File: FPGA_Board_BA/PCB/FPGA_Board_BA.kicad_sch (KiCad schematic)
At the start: 0 parts

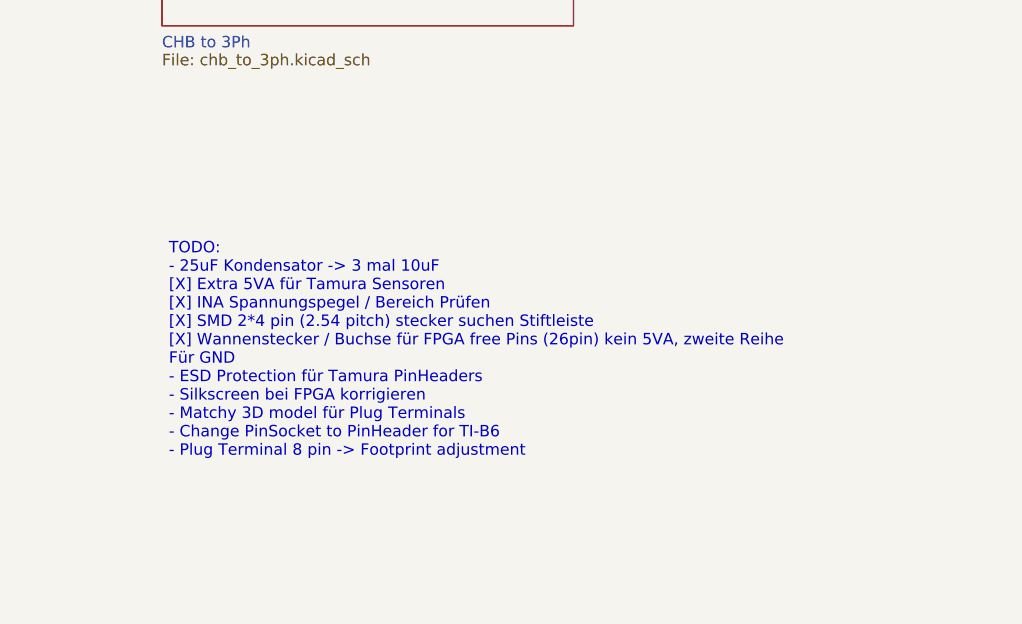
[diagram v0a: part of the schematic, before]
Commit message: Component placement ready. Waiting to meet with Leo
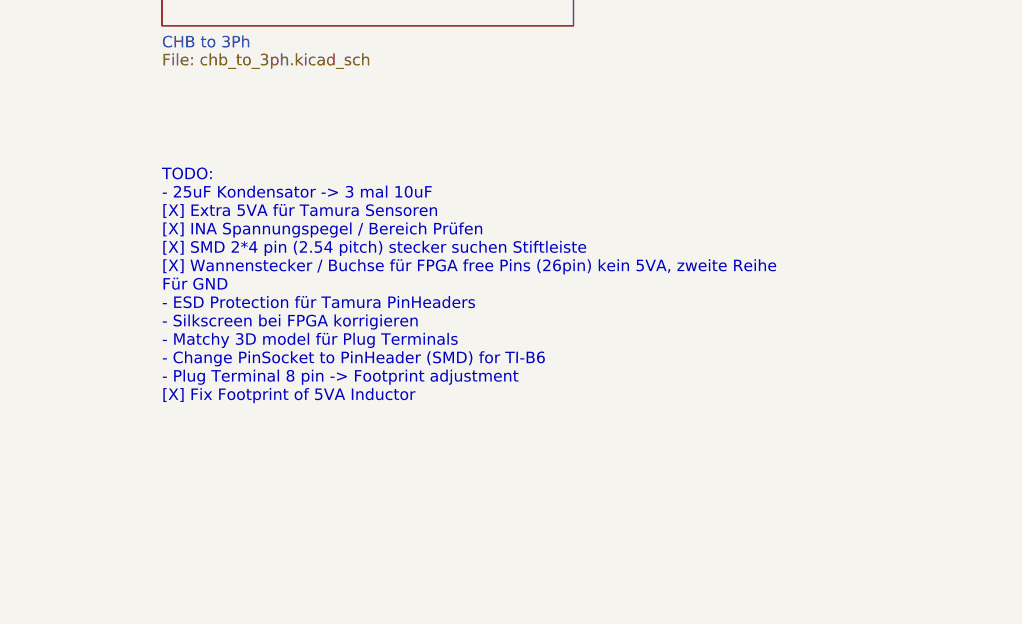
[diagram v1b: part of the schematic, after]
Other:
- note added: "TODO: - 25uF Kondensator -> 3 mal 10uF [X] Extra 5VA für Tamura Sensoren [X] INA Spannungspegel / Bereich Prüfen [X] SMD 2*4 pin (2.54 pitch) stecker suchen Stiftleiste [X] Wannenstecker / Buchse für FPGA free Pins (26pin) kein 5VA, zweite Reihe Für GND - ESD Protection für Tamura PinHeaders - Silkscreen bei FPGA korrigieren - Matchy 3D model für Plug Terminals - Change PinSocket to PinHeader (SM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"
- note removed: "TODO: - 25uF Kondensator -> 3 mal 10uF [X] Extra 5VA für Tamura Sensoren [X] INA Spannungspegel / Bereich Prüfen [X] SMD 2*4 pin (2.54 pitch) stecker suchen Stiftleiste [X] Wannenstecker / Buchse für FPGA free Pins (26pin) kein 5VA, zweite Reihe Für GND - ESD Protection für Tamura PinHeaders - Silkscreen bei FPGA korrigieren - Matchy 3D model für Plug Terminals - Change PinSocket to PinHeader for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"
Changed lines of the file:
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@@
 	(generator_version "9.0")
 	(paper "A3")
-	(text "TODO:\n- 25uF Kondensator -> 3 mal 10uF \n[X] Extra 5VA für Tamura Sensoren\n[X] INA Spannungspegel / Bereich Prüfen\n[X] SMD 2*4 pin (2.54 pitch) stecker suchen Stiftleiste\n[X] Wannenstecker / Buchse für FPGA free Pins (26pin) kein 5VA, zweite Reihe\nFür GND\n- ESD Protection für Tamura PinHeaders\n- Silkscreen bei FPGA korrigieren\n- Matchy 3D model für Plug Terminals\n- Change PinSocket to PinHeader for TI-B6\n- Plug Terminal 8 pin -> Footprint adjustment"
+	(text "TODO:\n- 25uF Kondensator -> 3 mal 10uF \n[X] Extra 5VA für Tamura Sensoren\n[X] INA Spannungspegel / Bereich Prüfen\n[X] SMD 2*4 pin (2.54 pitch) stecker suchen Stiftleiste\n[X] Wannenstecker / Buchse für FPGA free Pins (26pin) kein 5VA, zweite Reihe\nFür GND\n- ESD Protection für Tamura PinHeaders\n- Silkscreen bei FPGA korrigieren\n- Matchy 3D model für Plug Terminals\n- Change PinSocket to PinHeader (SMD) for TI-B6\n- Plug Terminal 8 pin -> Footprint adjustment\n[X] Fix Footprint of 5VA Inductor"
 		(exclude_from_sim no)
-		(at 328.422 239.268 0)
+		(at 327.66 232.156 0)
 		(effects
 			(font
